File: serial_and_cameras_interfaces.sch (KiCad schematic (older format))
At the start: 60 parts, among them J13 533980471, J15 533980471, J16 533980471, J17 533980471, J2 WE_68715014522, U16 NTS0102GT, U17 NTS0104PW,118, U18 MAX485EESA, U5 NTS0102GT, U6 PCA9547BS

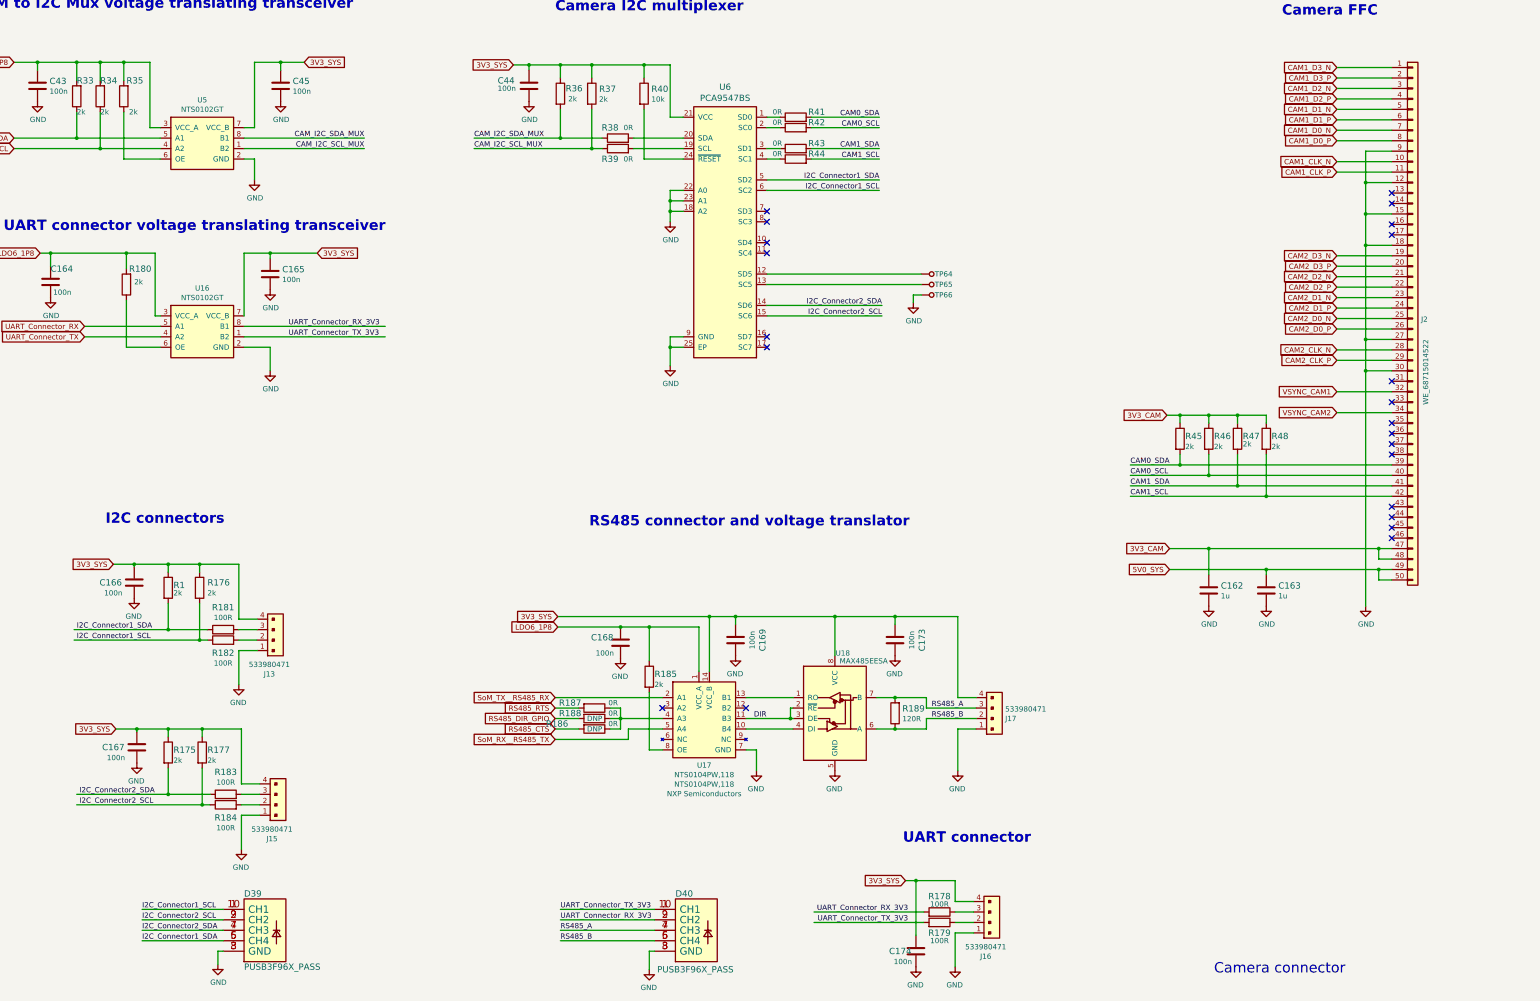
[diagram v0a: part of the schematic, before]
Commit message: Schematic cleanup
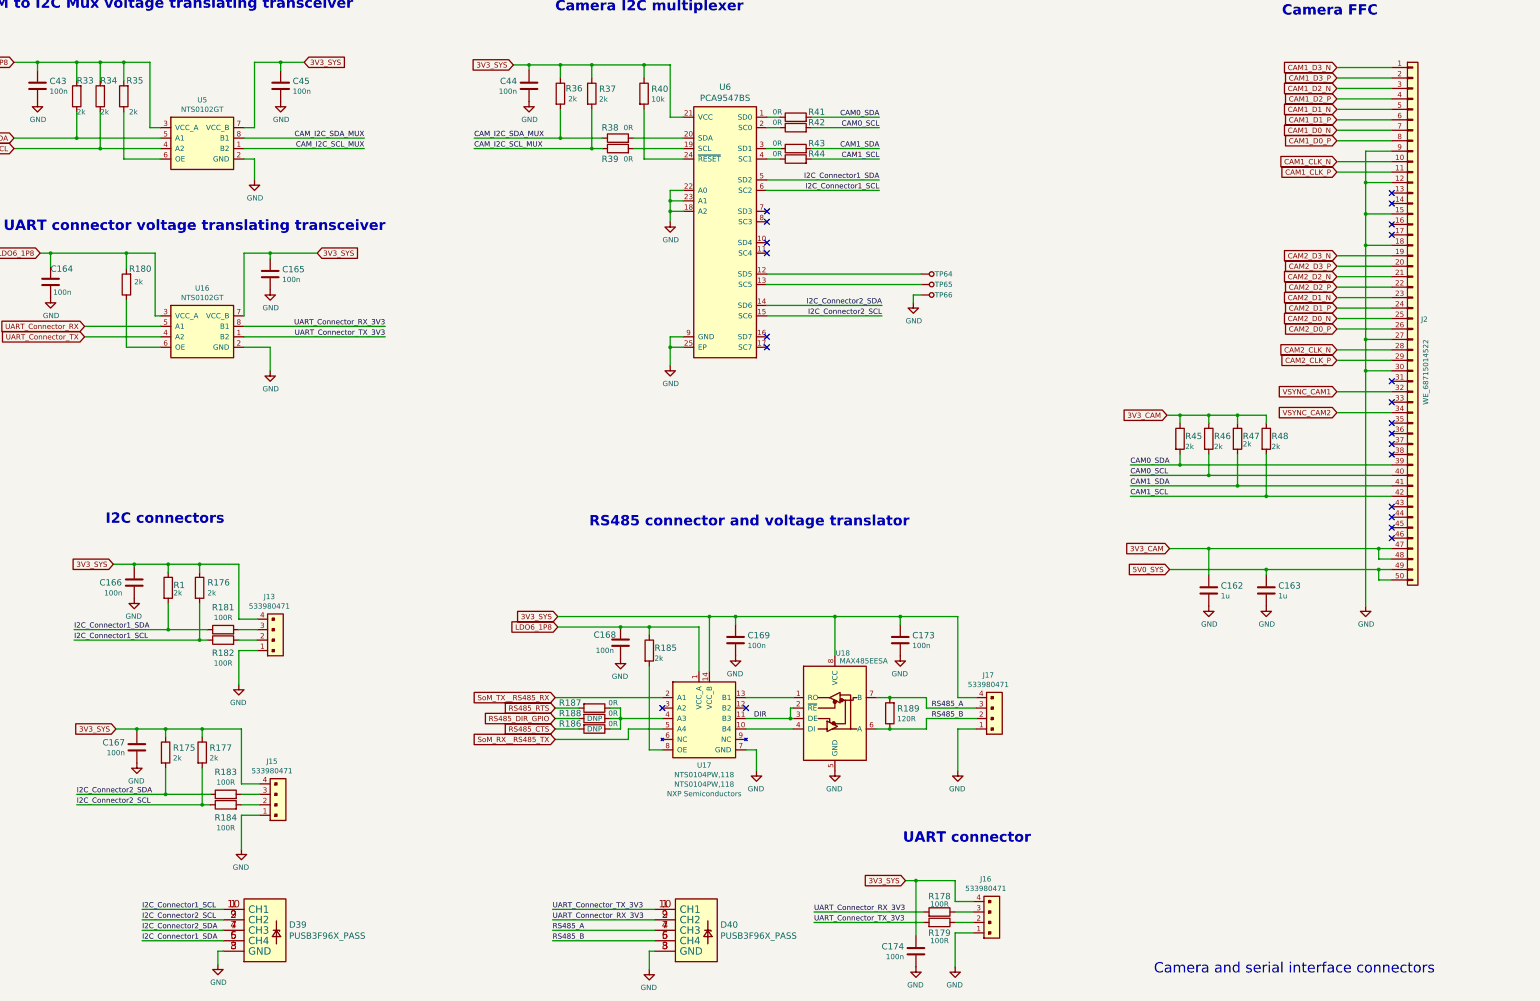
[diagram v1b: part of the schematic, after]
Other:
- note added: "Camera and serial interface connectors\n"
- note removed: "Camera connector\n"
- moved on the sheet: C173, R175, R185, R189
